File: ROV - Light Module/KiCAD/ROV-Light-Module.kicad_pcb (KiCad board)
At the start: 2 copper layers, 73.7 x 23.4 mm, 54 parts, among them J1 AVR UPDI Header, J4 Bottom - Middle, J6 Main In, J7 Bottom - Middle, J8 Middle - Top, J9 Middle - Top, U1 AL8805W5, U2 ATtiny1614-Arduino, U3 AP63205WU, U6 MAX3072E

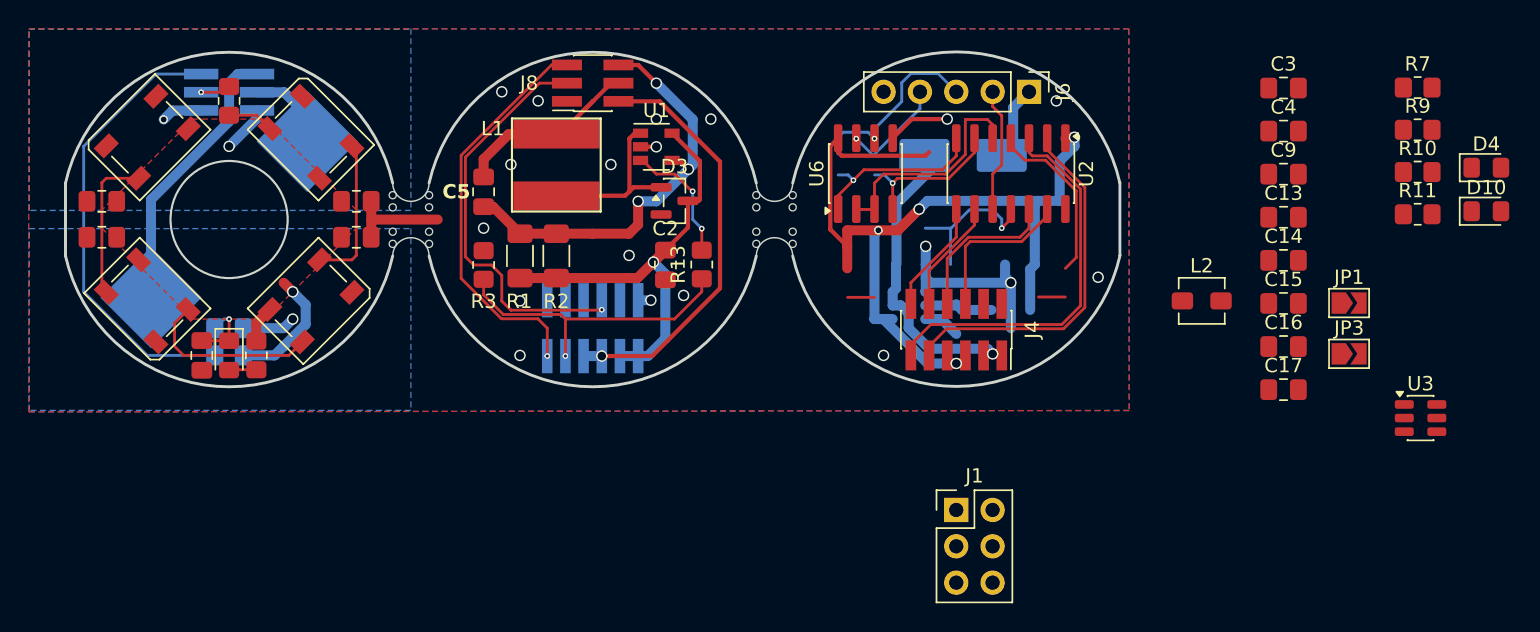
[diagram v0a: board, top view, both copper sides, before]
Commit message: updates
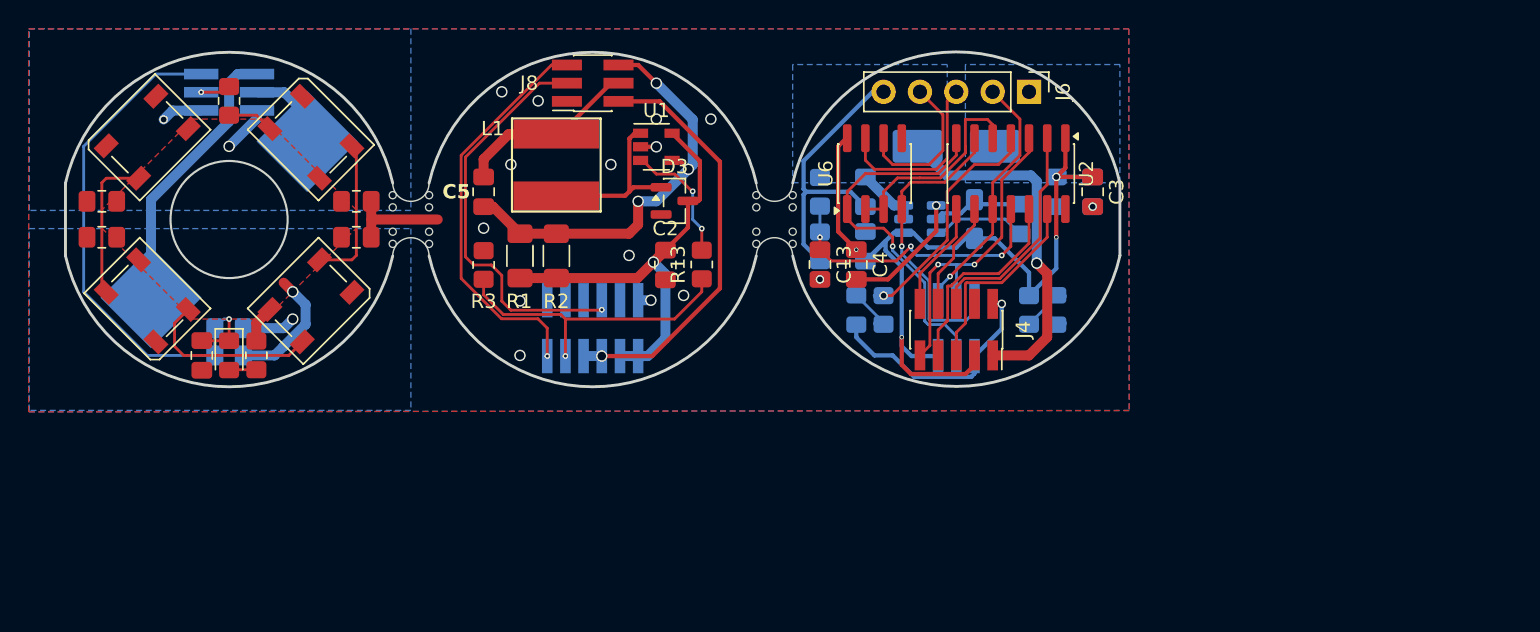
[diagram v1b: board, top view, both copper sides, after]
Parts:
- removed JP1: TX, Jumper:SolderJumper-2_P1.3mm_Open_TrianglePad1.0x1.5mm
- removed JP3: RX, Jumper:SolderJumper-2_P1.3mm_Open_TrianglePad1.0x1.5mm
- C14, C15, C16, C17, C9, D10, D4, L2, R10, R11, R7, R9, U3: moved to B.Cu
- C3: value 100nF -> 10pF
- J1: footprint Connector_PinHeader_2.54mm:PinHeader_2x03_P2.54mm_Vertical -> Connector_PinHeader_1.27mm:PinHeader_2x03_P1.27mm_Vertical_SMD; moved to B.Cu
- J4: value Bottom - Middle -> Conn_02x05_Odd_Even; footprint Connector_PinSocket_1.27mm:PinSocket_2x06_P1.27mm_Vertical_SMD -> Connector_PinSocket_1.27mm:PinSocket_2x05_P1.27mm_Vertical_SMD
- moved D4 45.1 mm to (183.5, 82.5), turned to 90 degrees
- moved R10 42.1 mm to (181.0, 78.1), turned to -90 degrees
- moved R9 42.0 mm to (181.0, 74.3), turned to -90 degrees
- moved R7 40.4 mm to (185.4, 82.5), turned to -90 degrees
- moved U3 37.6 mm to (188.0, 76.2)
- moved C13 32.6 mm to (181.0, 79.4), turned to -90 degrees
- moved C4 31.3 mm to (183.5, 79.4), turned to -90 degrees
- moved C17 30.9 mm to (184.2, 78.1), turned to -90 degrees
- moved D10 30.8 mm to (197.5, 82.5), turned to 90 degrees
- moved C14 29.6 mm to (184.2, 74.3), turned to 90 degrees
- moved R11 28.0 mm to (195.6, 82.5), turned to -90 degrees
- moved C15 19.3 mm to (194.9, 76.2), turned to -90 degrees
- moved C16 19.2 mm to (197.5, 74.3), turned to 90 degrees
- moved L2 16.9 mm to (191.8, 76.2), turned to -90 degrees
- moved C3 15.2 mm to (200.0, 74.3), turned to -90 degrees
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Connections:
- net Net-(D5-A) renamed V_Supply
- J4 pad 10: /Arduino Driver PCB/SCL -> /Arduino Driver PCB/SDA
- J4 pad 3: V_in -> +5V
- J4 pad 5: +5V -> /Arduino Driver PCB/NeoPixle
- J4 pad 6: /Arduino Driver PCB/NeoPixle -> /Arduino Driver PCB/LED_PWM
- J4 pad 7: +5V -> /Arduino Driver PCB/A9/D9
- J4 pad 8: /Arduino Driver PCB/A9/D9 -> /Arduino Driver PCB/SCL
- J4 pad 9: /Arduino Driver PCB/LED_PWM -> /Arduino Driver PCB/STATUS_LED
- J6 pad 3: /Arduino Driver PCB/Data_A -> /Arduino Driver PCB/Data_B
- J6 pad 4: /Arduino Driver PCB/Data_B -> /Arduino Driver PCB/Data_A
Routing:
- net GND: track 20.1 -> 60.8 mm
- net V_Supply: track 18.8 -> 0.00 mm, vias 2 -> 0
- net /Arduino Driver PCB/SERIAL_TX: track 12.8 -> 26.3 mm
- net /Arduino Driver PCB/SERIAL_RX: track 10.9 -> 21.3 mm
- net /Arduino Driver PCB/Vmeasure: track 10.2 -> 20.4 mm, vias 1 -> 3
- net /Arduino Driver PCB/UPDI: track 8.75 -> 17.7 mm, vias 0 -> 1
- net V_in: track 20.7 -> 29.3 mm
- net /Arduino Driver PCB/LED_PWM: track 24.1 -> 15.6 mm
- net /Arduino Driver PCB/Data_B: track 7.20 -> 12.8 mm, vias 1 -> 0
- net /Arduino Driver PCB/Builtin_LED: track 11.6 -> 16.2 mm, vias 0 -> 1
- net Net-(U3-BST): track 2.60 -> 6.22 mm
- net /Arduino Driver PCB/A9/D9: track 11.0 -> 14.5 mm
- net /Arduino Driver PCB/Data_A: track 13.3 -> 10.8 mm, vias 1 -> 0
- net /Arduino Driver PCB/NeoPixle: track 12.3 -> 14.3 mm
- net /Arduino Driver PCB/STATUS_LED: track 26.8 -> 24.8 mm, vias 0 -> 2
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- added copper zone on B.Cu, net V_Supply
- added copper zone on B.Cu, net V_in
